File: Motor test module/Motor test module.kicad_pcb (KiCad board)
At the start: 2 copper layers, 103.1 x 103.1 mm, 57 parts, among them J1 Conn_02x04_Counter_Clockwise, J2 Conn_02x04_Counter_Clockwise, J3 Conn_02x04_Counter_Clockwise, J4 Conn_02x04_Counter_Clockwise, J5 Conn_02x04_Counter_Clockwise, J6 Conn_02x04_Counter_Clockwise, J7 Conn_01x05_Male, J8 Screw_Terminal_01x02, J9 Screw_Terminal_01x02, SW1 SW_Push, U1 TPS63060, U10 ATA6560,1, U2 AP1017AEN, U3 AP1017AEN, U4 AP1017AEN, U5 AP1017AEN, U6 AP1017AEN, U7 AP1017AEN, U8 ATmega2560-16AU, U9 MCP2515-EST, Y1 16MHz, Y2 16MHz

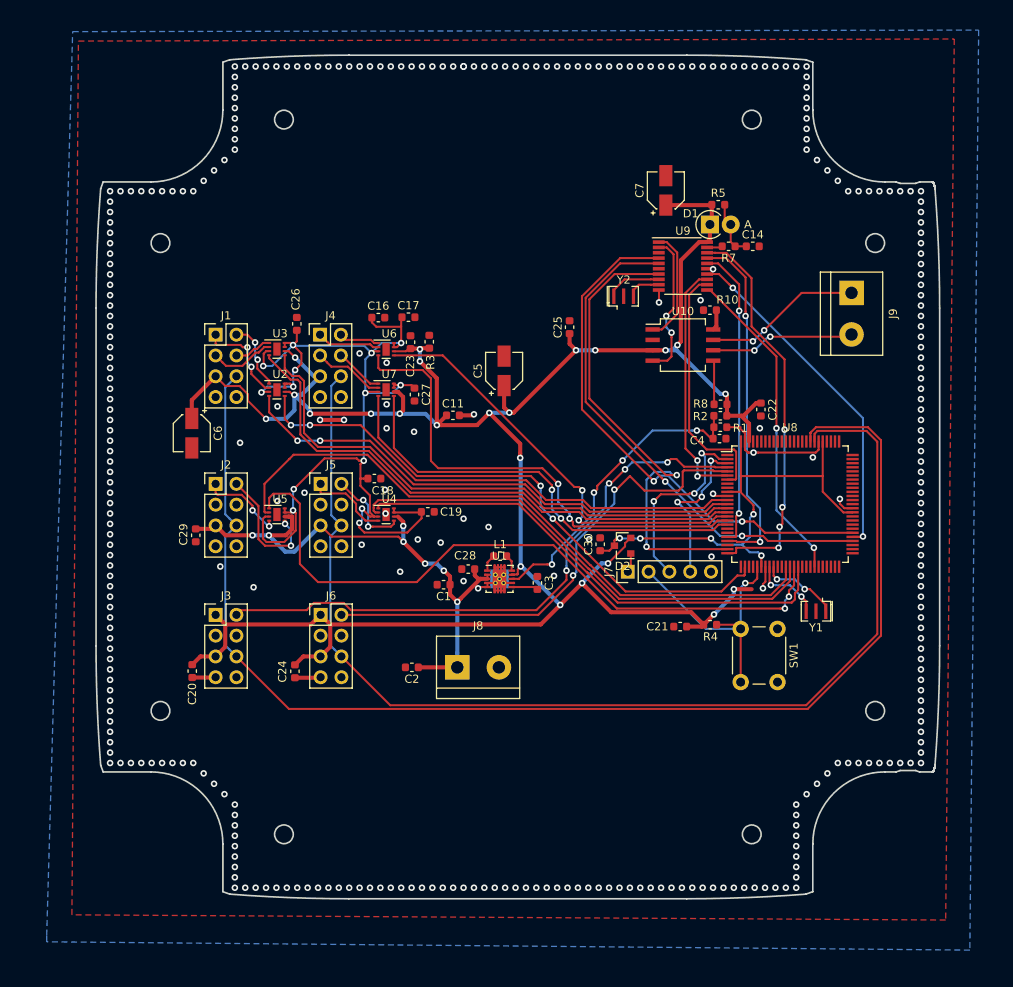
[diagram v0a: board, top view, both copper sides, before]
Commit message: Sixth draft of layout
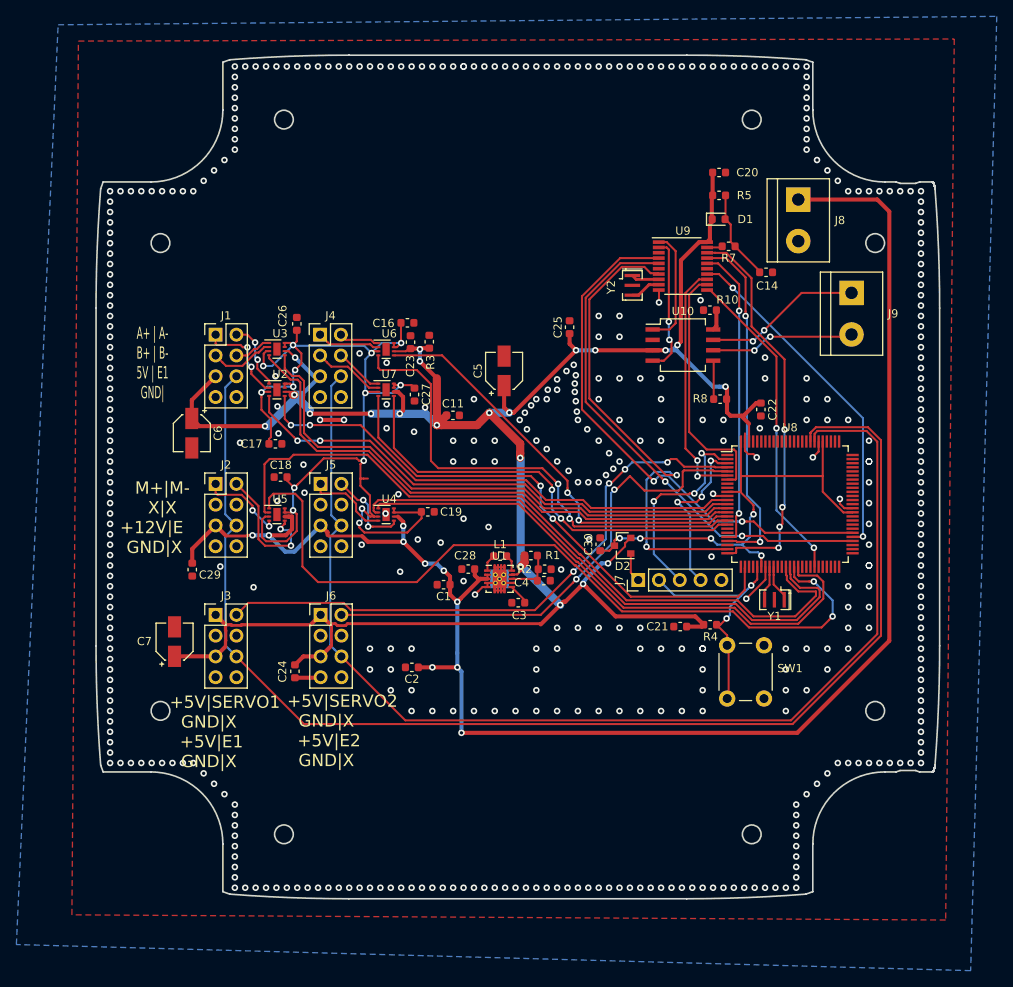
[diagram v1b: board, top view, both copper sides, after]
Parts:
- D1: footprint Diode_THT:D_DO-41_SOD81_P2.54mm_Vertical_AnodeUp -> Diode_SMD:D_0603_1608Metric
- moved C20 88.6 mm to (159.1, 65.4), turned to 0 degrees
- moved C7 81.5 mm to (92.6, 122.7)
- moved J8 70.7 mm to (168.8, 68.7), turned to 270 degrees
- moved R1 28.8 mm to (136.1, 112.2), turned to 0 degrees
- moved R2 27.6 mm to (137.8, 113.9)
- moved C4 27.6 mm to (137.7, 115.3)
- moved C17 22.4 mm to (104.9, 98.6)
- moved C18 11.5 mm to (105.5, 102.6), turned to 180 degrees
- moved Y1 5.27 mm to (165.9, 117.6)
- moved C29 4.21 mm to (94.7, 113.9)
- moved C16 3.61 mm to (121.0, 83.8)
- moved C14 3.57 mm to (164.8, 77.6)
- moved C3 3.36 mm to (134.6, 118.0), turned to 0 degrees
- moved SW1 2.60 mm to (164.6, 123.2)
- moved Y2 1.70 mm to (148.5, 79.2), turned to 270 degrees
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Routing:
- net +12V: track 69.1 -> 201.9 mm, vias 7 -> 10
- net Net-(C4-Pad2): track 37.8 -> 6.47 mm, vias 4 -> 0
- net M1-C: track 83.9 -> 95.2 mm
- net M1+C: track 78.7 -> 89.8 mm
- net GNDREF: track 43.0 -> 31.9 mm, vias 336 -> 457
- net M2+C: track 60.1 -> 69.8 mm
- net M2-C: track 60.7 -> 68.6 mm
- net +5V: track 284.7 -> 279.1 mm, vias 23 -> 21
- net Net-(U8-Pad34): track 9.72 -> 4.57 mm, vias 2 -> 0
- net Net-(U8-Pad33): track 8.64 -> 4.28 mm, vias 2 -> 0
- net Net-(C14-Pad1): track 6.98 -> 11.1 mm
- net +3V3: track 122.4 -> 126.1 mm
- net Net-(U9-Pad8): track 6.78 -> 3.42 mm
- net Rst: track 32.7 -> 29.8 mm, vias 1 -> 2
- net M2B-C: track 61.0 -> 62.6 mm
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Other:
- board text added: "+5V|SERVO1 GND|X +5V|E1 GND|X"
- board text added: "+5V|SERVO2 GND|X +5V|E2 GND|X"
- board text added: "A+ | A- B+ | B- 5V | E1 GND|"
- board text added: "M+|M- X|X +12V|E GND|X"
